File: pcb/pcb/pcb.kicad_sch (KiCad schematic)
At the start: 8 parts, among them J1 Connection 1, J2 Connection 2, J3 Motor1, J4 Motor2, J5 Motor4, J6 Motor3, J7 Bateria, J8 Motor3

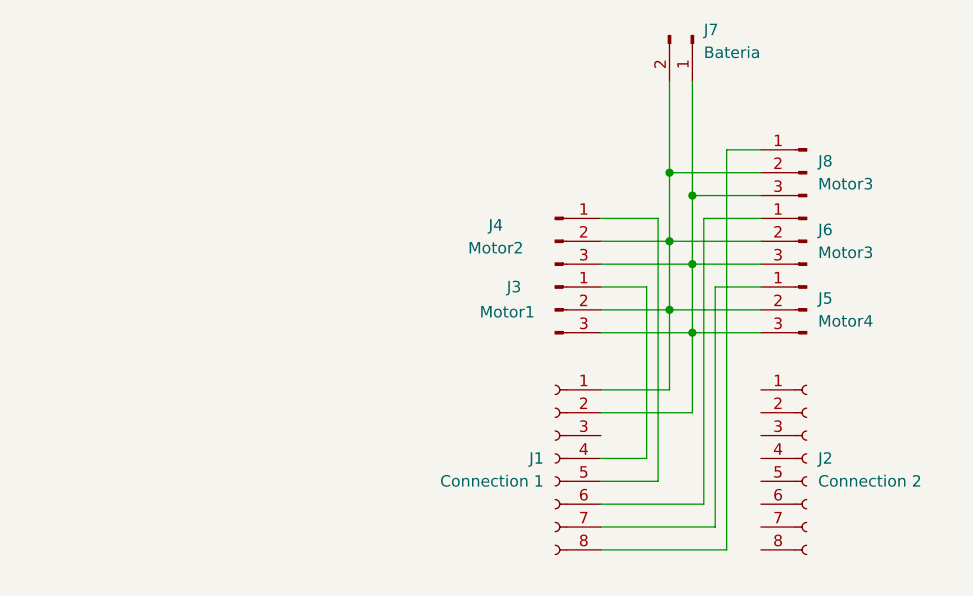
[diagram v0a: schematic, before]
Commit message: Update pcb and videos
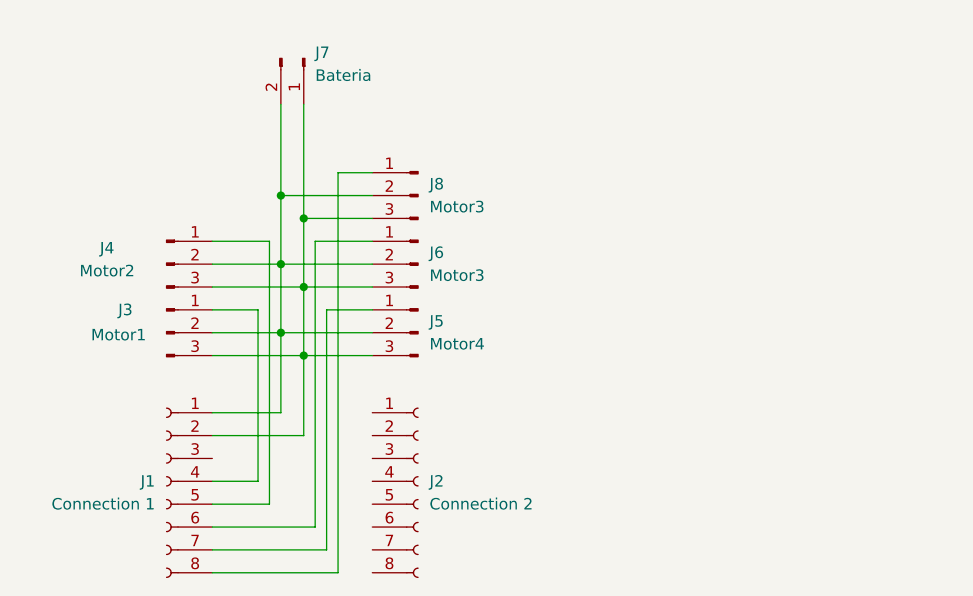
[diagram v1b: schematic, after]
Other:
- company: (none) -> forge-world-6798
- title: (none) -> Pcb Dednaugh
- moved on the sheet: J1, J2, J3, J4, J5, J6, J7, J8
